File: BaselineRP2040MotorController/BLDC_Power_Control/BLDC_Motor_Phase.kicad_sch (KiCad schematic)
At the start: 28 parts, among them Q3 Q_PNP_BEC, U10 INA240A1D, U9 EG3113

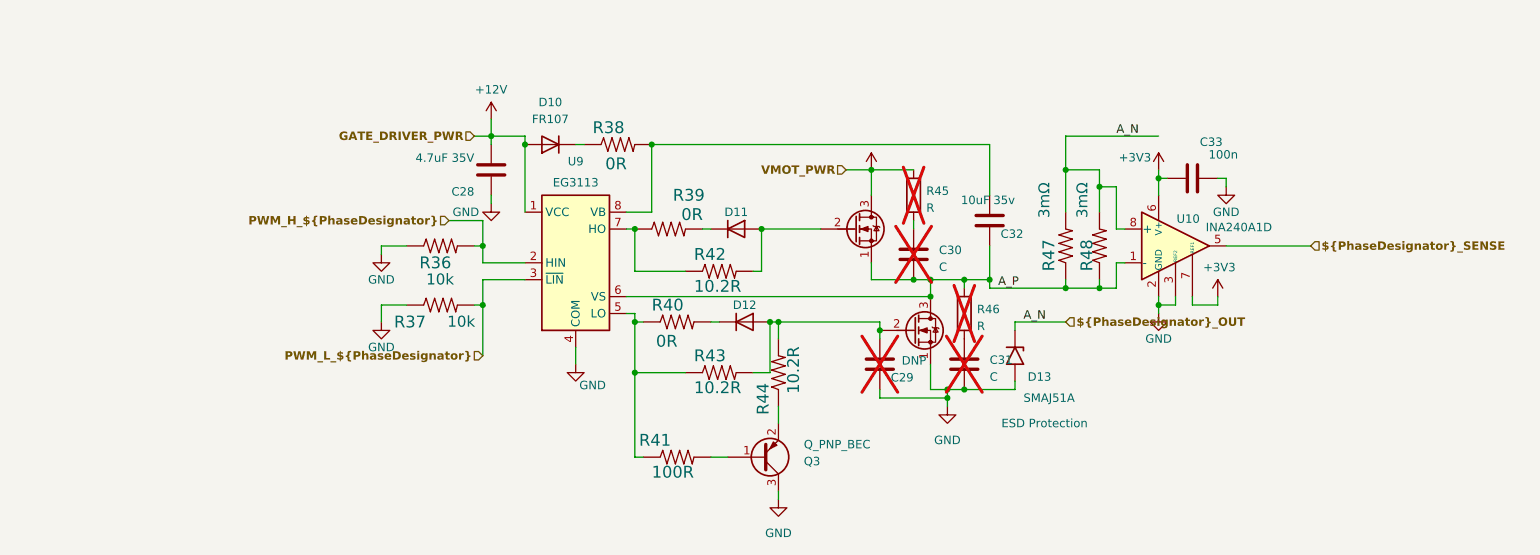
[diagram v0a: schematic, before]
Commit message: Erhhhhrh
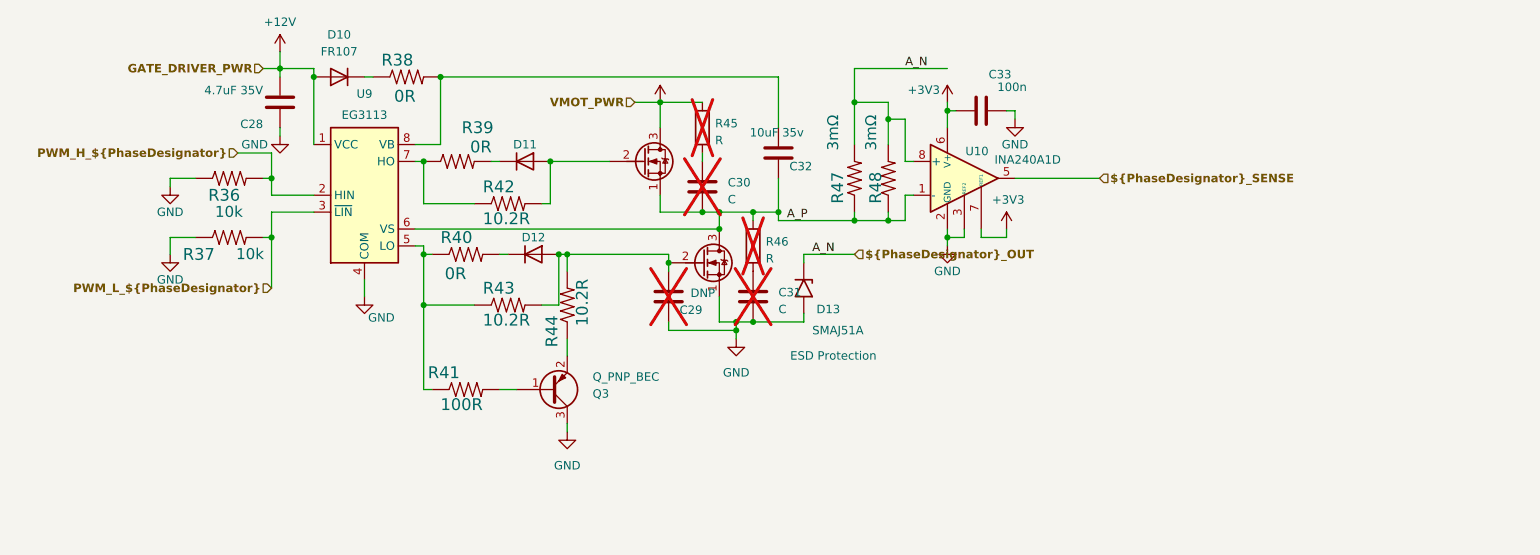
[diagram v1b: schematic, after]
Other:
- moved on the sheet: C28, C29, C30, C31, C32, C33, D10, D11, D12, D13, Q3, R36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
